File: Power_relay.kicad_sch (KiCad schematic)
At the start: 8 parts, among them K1 HE1AN-W-DC12V-Y6, Q5 Q_NMOS_GSD

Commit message: update art work
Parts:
- K1: footprint RDC_generic:HE1AN-W-DC12V-Y6 -> RDC_generic:HE1AN-W-DC12V-Y6+Y5
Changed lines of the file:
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@@
       (effects (font (size 1.27 1.27)) (justify left))
     )
-    (property "Footprint" "RDC_generic:HE1AN-W-DC12V-Y6" (at 118.11 68.58 0)
+    (property "Footprint" "RDC_generic:HE1AN-W-DC12V-Y6+Y5" (at 118.11 68.58 0)
       (effects (font (size 1.27 1.27)) hide)
     )

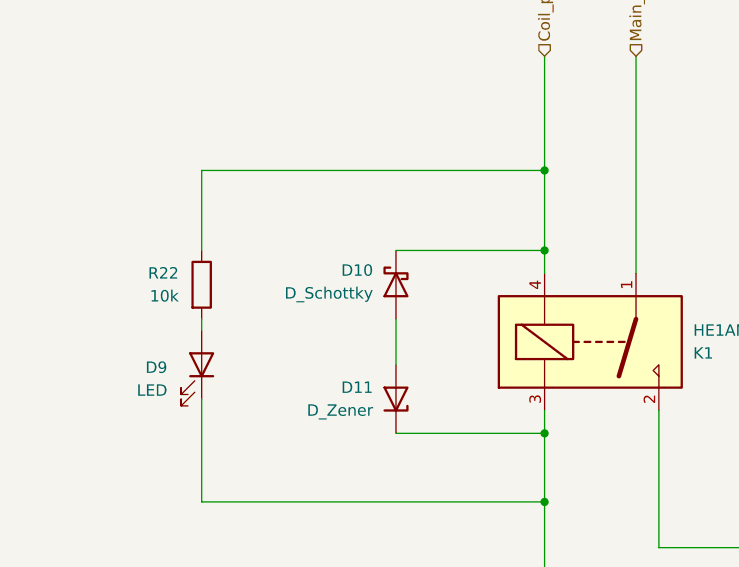
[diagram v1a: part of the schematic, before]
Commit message: アートワークのほとんど終わり
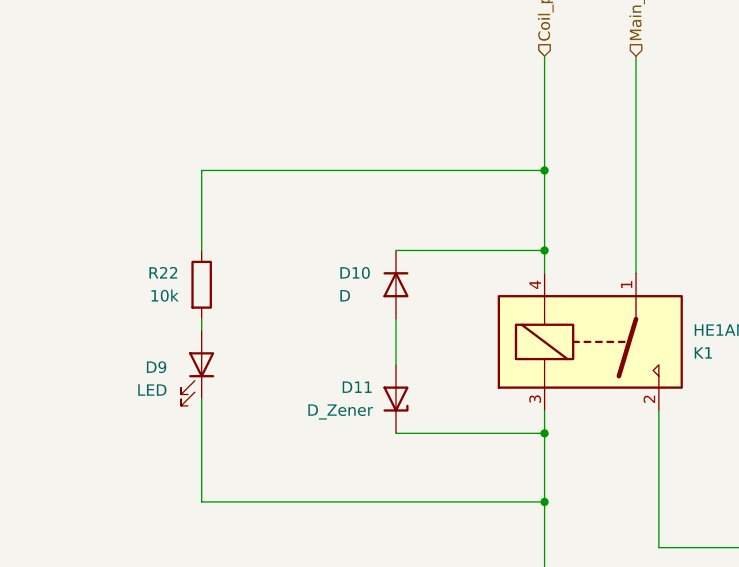
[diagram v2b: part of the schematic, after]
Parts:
- D10: value D_Schottky -> D; symbol Device:D_Schottky -> Device:D; LCSC C22466347 -> C18199085
- D11: footprint Diode_SMD:D_SOD-123F -> Diode_SMD:D_SMA; LCSC (none) -> C19077489
- D9: footprint LED_SMD:LED_0603_1608Metric_Pad1.05x0.95mm_HandSolder -> LED_SMD:LED_0603_1608Metric; LCSC (none) -> C2286
- Q5: LCSC (none) -> C7420346
- R22, R24: LCSC (none) -> C25744
- R23: LCSC (none) -> C25076
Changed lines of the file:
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@@
+      (effects (font (size 1.27 1.27)) hide)
+    )
+    (property "LCSC" "C25744" (at 101.6 124.46 0)
       (effects (font (size 1.27 1.27)) hide)
     )
@@
     )
     (property "Datasheet" "~" (at 110.49 118.11 0)
+      (effects (font (size 1.27 1.27)) hide)
+    )
+    (property "LCSC" "C7420346" (at 110.49 118.11 0)
       (effects (font (size 1.27 1.27)) hide)
     )
@@
       (effects (font (size 1.27 1.27)) hide)
     )
+    (property "LCSC" "C25076" (at 93.98 118.11 0)
+      (effects (font (size 1.27 1.27)) hide)
+    )
     (pin "2")
     (pin "1")
@@
       (effects (font (size 1.27 1.27)) (justify right))
     )
-    (property "Footprint" "Diode_SMD:D_SOD-123F" (at 96.52 85.09 0)
+    (property "Footprint" "Diode_SMD:D_SMA" (at 96.52 85.09 0)
       (effects (font (size 1.27 1.27)) hide)
     )
     (property "Datasheet" "~" (at 96.52 85.09 0)
+      (effects (font (size 1.27 1.27)) hide)
+    )
+    (property "LCSC" "C19077489" (at 96.52 85.09 0)
       (effects (font (size 1.27 1.27)) hide)
     )
@@
       (effects (font (size 1.27 1.27)) (justify right))
     )
-    (property "Footprint" "LED_SMD:LED_0603_1608Metric_Pad1.05x0.95mm_HandSolder" (at 74.93 81.28 0)
+    (property "Footprint" "LED_SMD:LED_0603_1608Metric" (at 74.93 81.28 0)
       (effects (font (size 1.27 1.27)) hide)
     )
     (property "Datasheet" "~" (at 74.93 81.28 0)
+      (effects (font (size 1.27 1.27)) hide)
+    )
+    (property "LCSC" "C2286" (at 74.93 81.28 0)
       (effects (font (size 1.27 1.27)) hide)
     )
@@
       (effects (font (size 1.27 1.27)) hide)
     )
+    (property "LCSC" "C25744" (at 74.93 72.39 0)
+      (effects (font (size 1.27 1.27)) hide)
+    )
     (pin "2")
     (pin "1")
@@
     )
   )
-  (symbol (lib_id "Device:D_Schottky") (at 96.52 72.39 90) (mirror x) (unit 1)
-    (in_bom yes) (on_board yes) (dnp no) (fields_autoplaced)
-    (property "Reference" "D10" (at 93.98 70.8025 90)
-      (effects (font (size 1.27 1.27)) (justify left))
+  (symbol (lib_id "Device:D") (at 96.52 72.39 90) (mirror x) (unit 1)
+    (in_bom yes) (on_board yes) (dnp no)
+    (property "Reference" "D10" (at 90.17 71.12 90)
+      (effects (font (size 1.27 1.27)) (justify right))
     )
-    (property "Value" "D_Schottky" (at 93.98 73.3425 90)
-      (effects (font (size 1.27 1.27)) (justify left))
+    (property "Value" "D" (at 90.17 73.66 90)
+      (effects (font (size 1.27 1.27)) (justify right))
     )
     (property "Footprint" "Diode_SMD:D_SOD-123F" (at 96.52 72.39 0)
@@
       (effects (font (size 1.27 1.27)) hide)
     )
-    (property "LCSC" "C22466347" (at 96.52 72.39 0)
+    (property "LCSC" "C18199085" (at 96.52 72.39 0)
       (effects (font (size 1.27 1.27)) hide)
     )
+    (property "Sim.Device" "D" (at 96.52 72.39 0)
+      (effects (font (size 1.27 1.27)) hide)
+    )
+    (property "Sim.Pins" "1=K 2=A" (at 96.52 72.39 0)
+      (effects (font (size 1.27 1.27)) hide)
+    )
